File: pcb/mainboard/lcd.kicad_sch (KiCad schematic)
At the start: 3 parts, among them J503 FH12-40S-0.5SH, U504 SM351LT

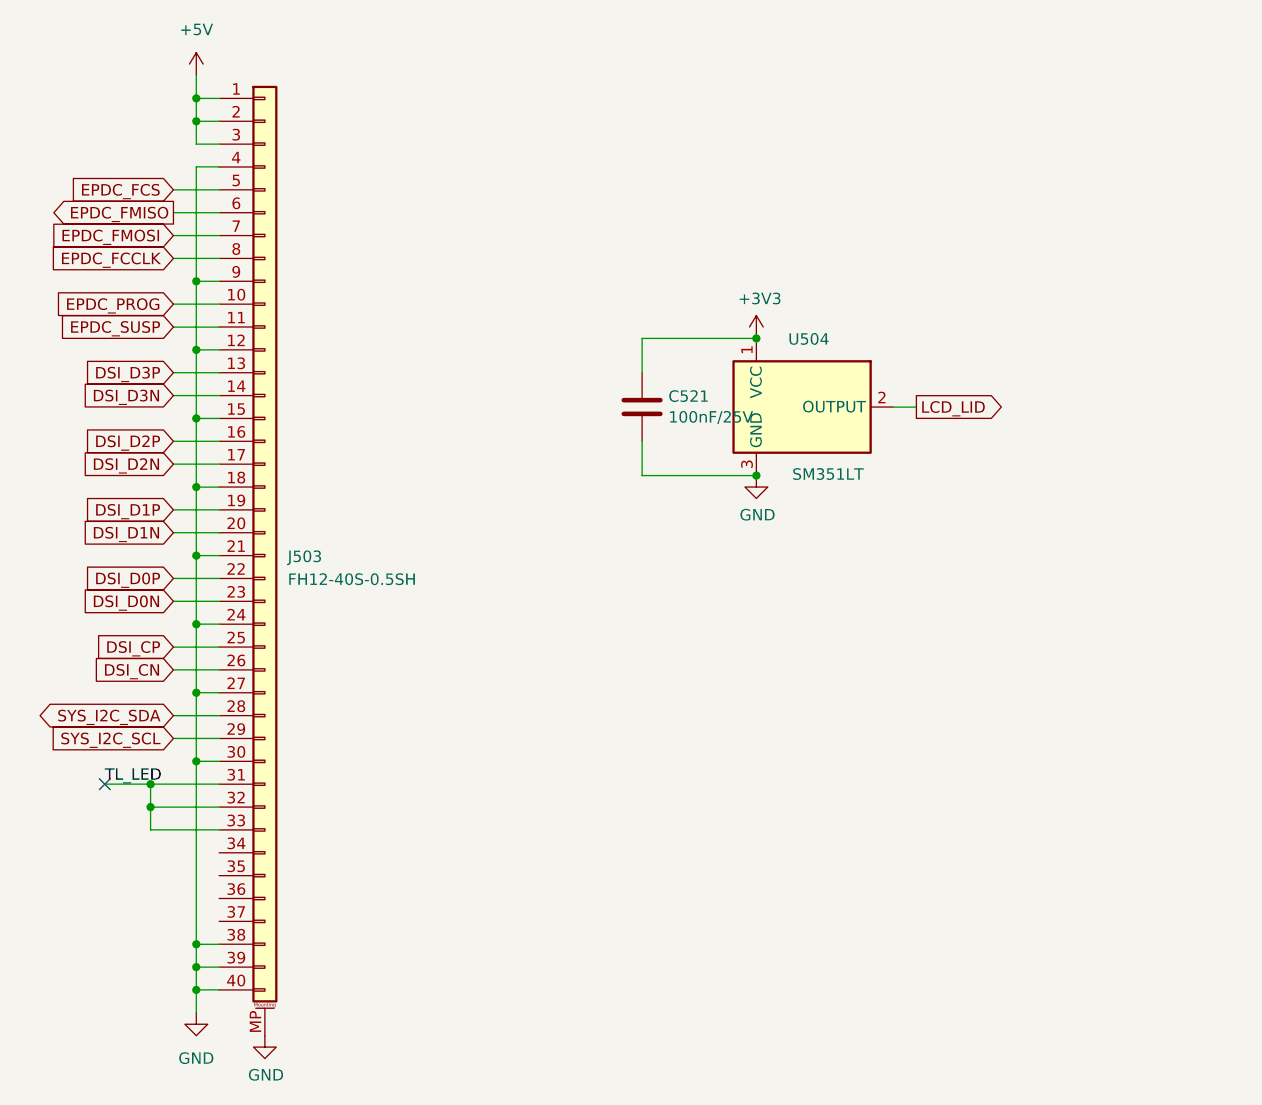
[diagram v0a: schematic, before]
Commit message: pcb: r0.1 mb routing done
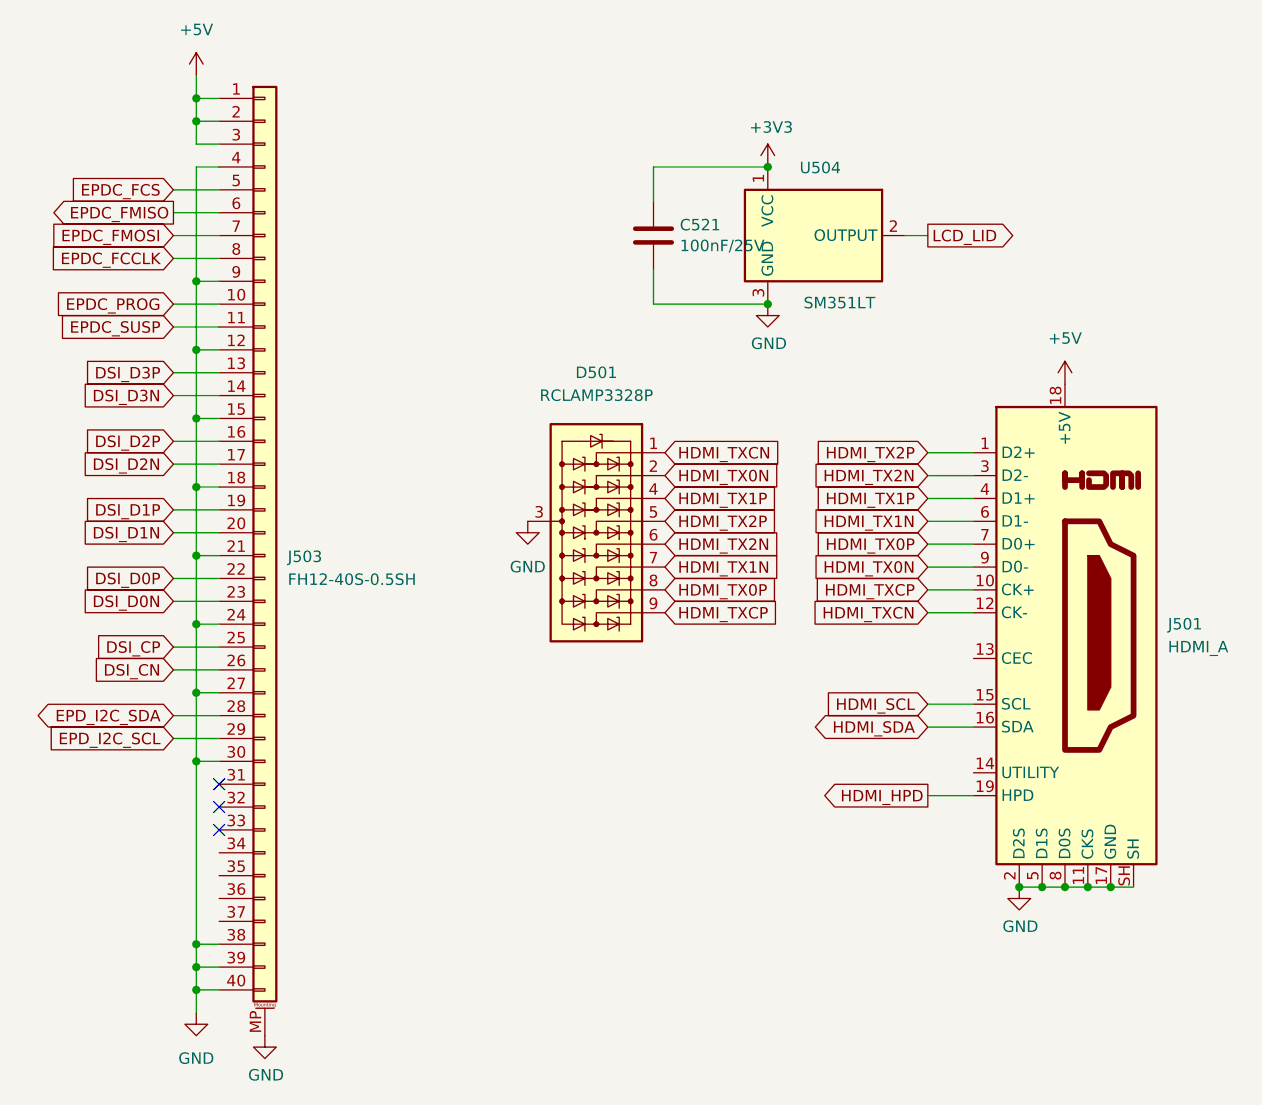
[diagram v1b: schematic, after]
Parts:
- added D501: RCLAMP3328P, Package_DFN_QFN:UDFN-9_1.0x3.8mm_P0.5mm, symbol Power_Protection:RCLAMP3328P
- added J501: HDMI_A, footprints:HDMI-D-Stripped, symbol Connector:HDMI_A
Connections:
- net +5V: now also J501.18 (+5V)
- net GND: now also D501.3 (A), J501.11 (CKS), J501.17 (GND), J501.2 (D2S), J501.5 (D1S), J501.8 (D0S), J501.SH
- net SYS_I2C_SCL renamed EPD_I2C_SCL
- net SYS_I2C_SDA renamed EPD_I2C_SDA
- removed net TL_LED: J503.31 (Pin_31), J503.32 (Pin_32), J503.33 (Pin_33)
- new net HDMI_HPD: J501.19 (HPD)
- new net HDMI_SCL: J501.15 (SCL)
- new net HDMI_SDA: J501.16 (SDA)
- new net HDMI_TX0N: D501.2 (K2), J501.9 (D0-)
- new net HDMI_TX0P: D501.8 (K7), J501.7 (D0+)
- new net HDMI_TX1N: D501.7 (K6), J501.6 (D1-)
- new net HDMI_TX1P: D501.4 (K3), J501.4 (D1+)
- new net HDMI_TX2N: D501.6 (K5), J501.3 (D2-)
- new net HDMI_TX2P: D501.5 (K4), J501.1 (D2+)
- new net HDMI_TXCN: D501.1 (K1), J501.12 (CK-)
- new net HDMI_TXCP: D501.9 (K8), J501.10 (CK+)
- no-connect marks 1 -> 3
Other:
- moved on the sheet: C521, U504
